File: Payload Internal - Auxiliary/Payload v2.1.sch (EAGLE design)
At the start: 11 parts, among them J30 M80-866XXXX, J31 M80-866XXXX

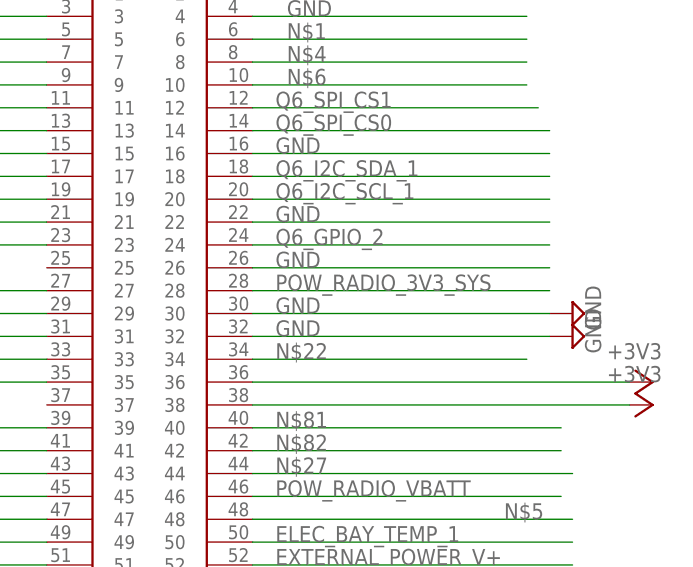
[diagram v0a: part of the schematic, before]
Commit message: [PAYLOAD-INT] added h2 pin 26 and pin 28 short (to match actual PCB)
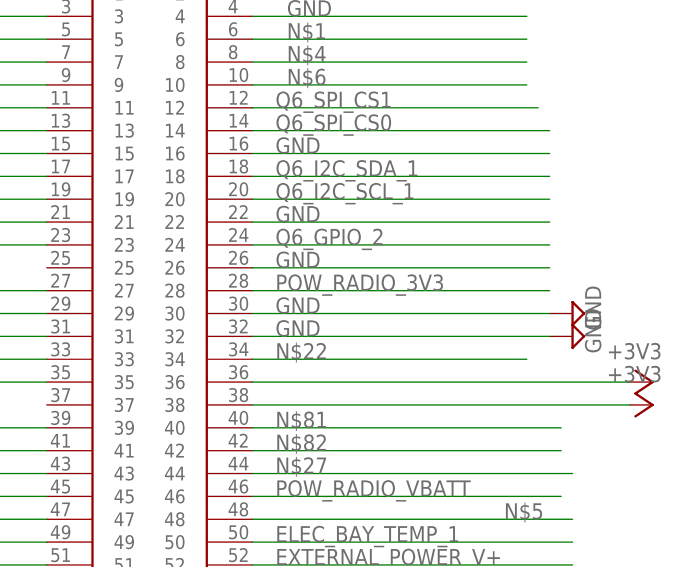
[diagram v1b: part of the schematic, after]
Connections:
- removed net POW_RADIO_3V3_SYS: H2.28
- net POW_RADIO_3V3: now also H2.28
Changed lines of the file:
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@@
 <setting verticaltext="up"/>
 </settings>
-<grid distance="1.27" unitdist="mm" unit="mm" style="lines" multiple="1" display="no" altdistance="0.01" altunitdist="inch" altunit="mm"/>
+<grid distance="0.1" unitdist="inch" unit="inch" style="lines" multiple="1" display="no" altdistance="0.01" altunitdist="inch" altunit="inch"/>
 <layers>
 <layer number="1" name="Top" color="4" fill="1" visible="no" active="no"/>
@@
 <label x="-203.2" y="68.58" size="1.778" layer="95"/>
 </segment>
-</net>
-<net name="POW_RADIO_3V3_SYS" class="0">
 <segment>
 <pinref part="H2" gate="G$1" pin="28"/>
